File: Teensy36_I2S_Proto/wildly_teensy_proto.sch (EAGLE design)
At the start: 22 parts, among them CON1 MIKROE_BUS_CONN, SW1 SPST_TACT-KMR2, X1 ANTENNA

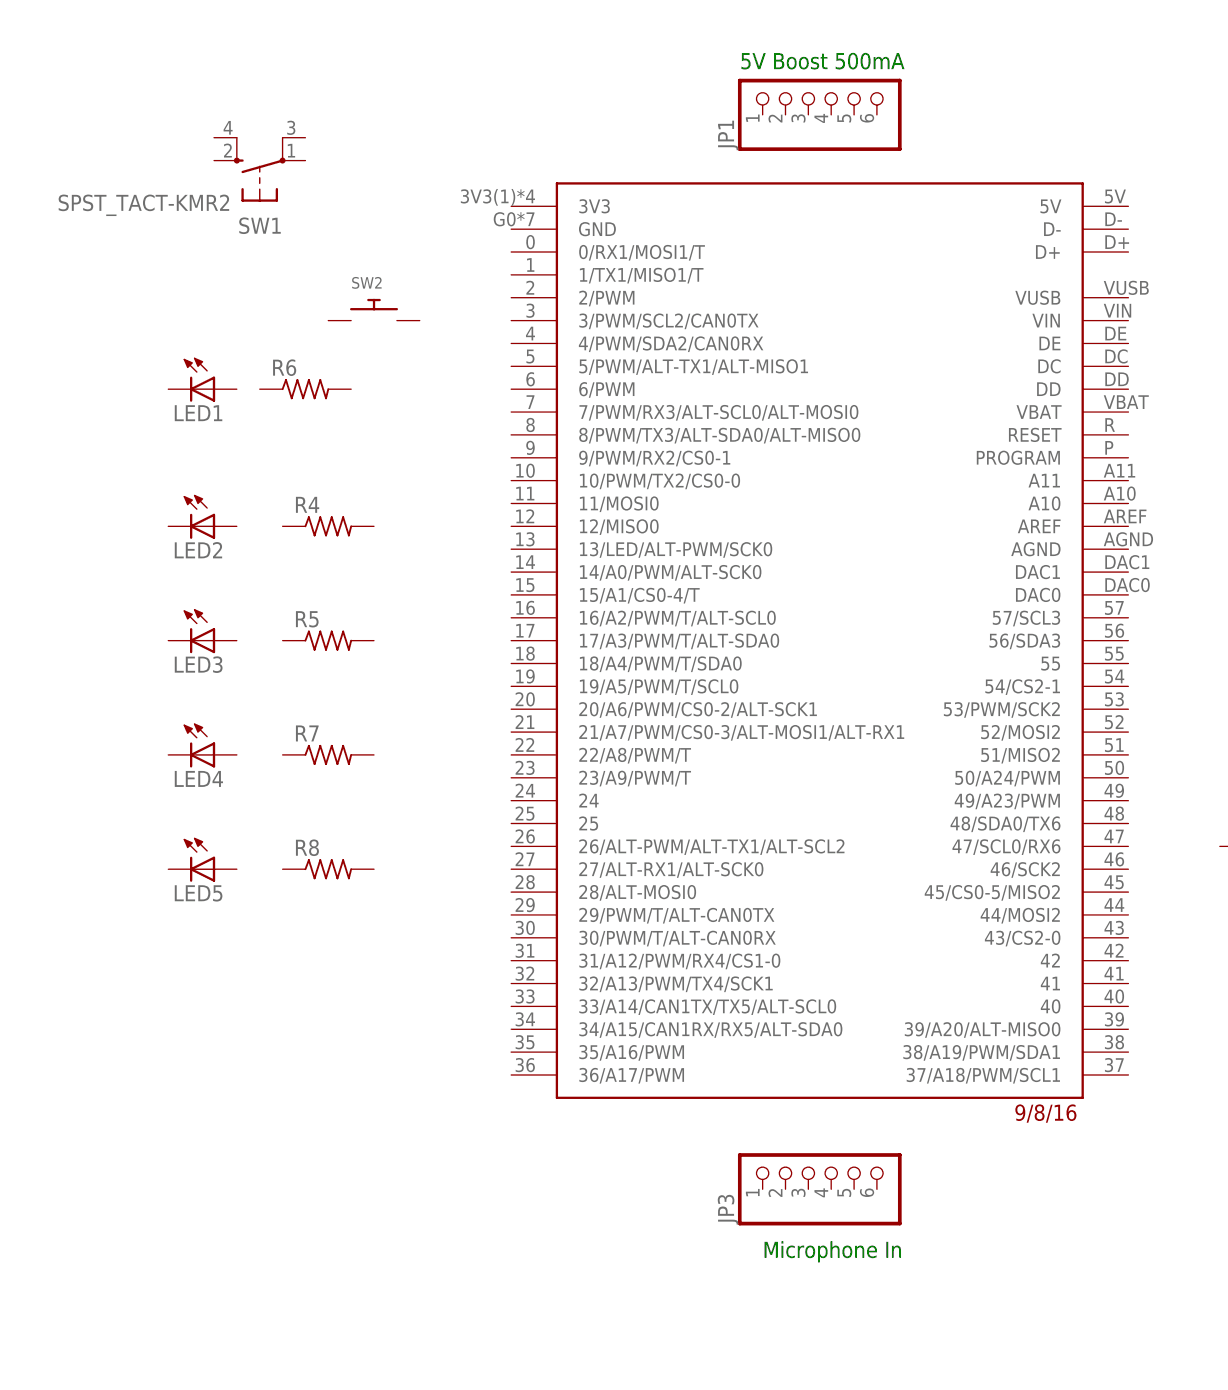
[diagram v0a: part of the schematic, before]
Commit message: Add files via upload
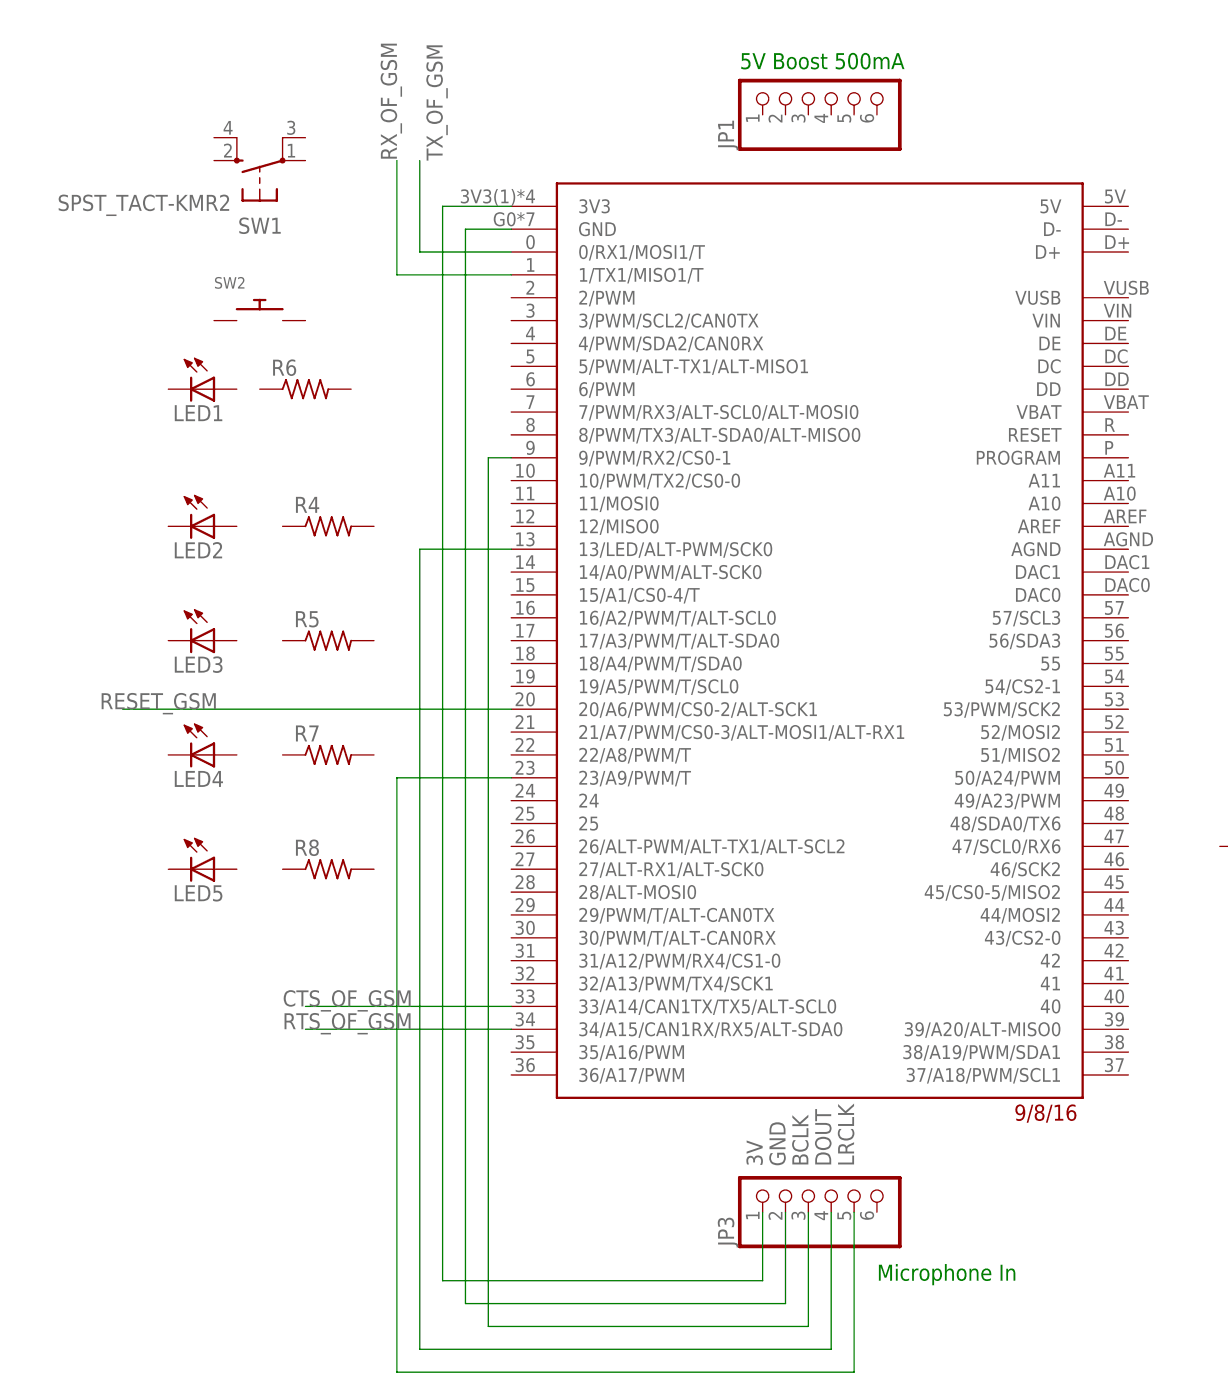
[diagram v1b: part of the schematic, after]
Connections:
- new net 3V: JP3.1, U$1.3V3
- new net BCLK: JP3.3, U$1.9/PWM/RX2/CS0-1
- new net CTS_OF_GSM: U$1.33/A14/CAN1TX/TX5/ALT-SCL0
- new net DOUT: JP3.4, U$1.13/LED/ALT-PWM/SCK0
- new net GND: JP3.2, U$1.GND
- new net LRCLK: JP3.5, U$1.23/A9/PWM/T
- new net RESET_GSM: U$1.20/A6/PWM/CS0-2/ALT-SCK1
- new net RTS_OF_GSM: U$1.34/A15/CAN1RX/RX5/ALT-SDA0
- new net RX_OF_GSM: U$1.1/TX1/MISO1/T
- new net TX_OF_GSM: U$1.0/RX1/MOSI1/T
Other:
- moved on the sheet: JP3, SW2
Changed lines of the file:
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@@
 <?xml version="1.0" encoding="utf-8"?>
 <!DOCTYPE eagle SYSTEM "eagle.dtd">
-<eagle version="9.3.0">
+<eagle version="9.2.2">
 <drawing>
 <settings>
@@
 <setting verticaltext="up"/>
 </settings>
-<grid distance="0.1" unitdist="inch" unit="inch" style="lines" multiple="1" display="no" altdistance="0.01" altunitdist="inch" altunit="inch"/>
+<grid distance="0.1" unitdist="inch" unit="inch" style="dots" multiple="1" display="yes" altdistance="0.01" altunitdist="inch" altunit="inch"/>
 <layers>
 <layer number="1" name="Top" color="4" fill="1" visible="no" active="no"/>
@@
 <sheet>
 <plain>
-<text x="58.42" y="-25.4" size="1.778" layer="91">Microphone In</text>
+<text x="71.12" y="-27.94" size="1.778" layer="91">Microphone In</text>
 <text x="55.88" y="106.68" size="1.778" layer="91">5V Boost 500mA</text>
 <text x="129.54" y="10.16" size="1.778" layer="91">5V Boost 1A</text>
@@
 <attribute name="VALUE" x="-0.635" y="92.71" size="1.778" layer="96" rot="R180"/>
 </instance>
-<instance part="SW2" gate="G$1" x="15.24" y="78.74" smashed="yes">
-<attribute name="NAME" x="12.7" y="82.296" size="1.27" layer="95"/>
-<attribute name="VALUE" x="12.7" y="76.454" size="1.27" layer="96"/>
+<instance part="SW2" gate="G$1" x="2.54" y="78.74" smashed="yes">
+<attribute name="NAME" x="-2.54" y="82.296" size="1.27" layer="95"/>
+<attribute name="VALUE" x="0" y="76.454" size="1.27" layer="96"/>
 </instance>
 <instance part="JP2" gate="G$1" x="137.16" y="15.24" smashed="yes" rot="R270">
@@
 <attribute name="VALUE" x="121.92" y="21.59" size="1.778" layer="96" rot="R270"/>
 </instance>
-<instance part="JP3" gate="A" x="66.04" y="-15.24" smashed="yes" rot="R90">
-<attribute name="NAME" x="55.245" y="-21.59" size="1.778" layer="95" rot="R90"/>
-<attribute name="VALUE" x="76.2" y="-21.59" size="1.778" layer="96" rot="R90"/>
+<instance part="JP3" gate="A" x="66.04" y="-17.78" smashed="yes" rot="R90">
+<attribute name="NAME" x="55.245" y="-24.13" size="1.778" layer="95" rot="R90"/>
+<attribute name="VALUE" x="76.2" y="-24.13" size="1.778" layer="96" rot="R90"/>
 </instance>
 <instance part="R8" gate="G$1" x="10.16" y="17.78" smashed="yes">
@@
 </segment>
 </net>
+<net name="3V" class="0">
+<segment>
+<pinref part="JP3" gate="A" pin="1"/>
+<wire x1="58.42" y1="-20.32" x2="58.42" y2="-27.94" width="0.1524" layer="91"/>
+<wire x1="58.42" y1="-27.94" x2="22.86" y2="-27.94" width="0.1524" layer="91"/>
+<wire x1="22.86" y1="-27.94" x2="22.86" y2="91.44" width="0.1524" layer="91"/>
+<pinref part="U$1" gate="G$1" pin="3V3"/>
+<wire x1="22.86" y1="91.44" x2="30.48" y2="91.44" width="0.1524" layer="91"/>
+<label x="58.42" y="-15.24" size="1.778" layer="95" rot="R90"/>
+</segment>
+</net>
+<net name="GND" class="0">
+<segment>
+<pinref part="JP3" gate="A" pin="2"/>
+<wire x1="60.96" y1="-20.32" x2="60.96" y2="-30.48" width="0.1524" layer="91"/>
+<wire x1="60.96" y1="-30.48" x2="25.4" y2="-30.48" width="0.1524" layer="91"/>
+<wire x1="25.4" y1="-30.48" x2="25.4" y2="88.9" width="0.1524" layer="91"/>
+<pinref part="U$1" gate="G$1" pin="GND"/>
+<wire x1="25.4" y1="88.9" x2="30.48" y2="88.9" width="0.1524" layer="91"/>
+<label x="60.96" y="-15.24" size="1.778" layer="95" rot="R90"/>
+</segment>
+</net>
+<net name="BCLK" class="0">
+<segment>
+<pinref part="JP3" gate="A" pin="3"/>
+<wire x1="63.5" y1="-20.32" x2="63.5" y2="-33.02" width="0.1524" layer="91"/>
+<wire x1="63.5" y1="-33.02" x2="27.94" y2="-33.02" width="0.1524" layer="91"/>
+<pinref part="U$1" gate="G$1" pin="9/PWM/RX2/CS0-1"/>
+<wire x1="27.94" y1="-33.02" x2="27.94" y2="63.5" width="0.1524" layer="91"/>
+<wire x1="27.94" y1="63.5" x2="30.48" y2="63.5" width="0.1524" layer="91"/>
+<label x="63.5" y="-15.24" size="1.778" layer="95" rot="R90"/>
+</segment>
+</net>
+<net name="DOUT" class="0">
+<segment>
+<pinref part="JP3" gate="A" pin="4"/>
+<wire x1="66.04" y1="-20.32" x2="66.04" y2="-35.56" width="0.1524" layer="91"/>
+<wire x1="66.04" y1="-35.56" x2="20.32" y2="-35.56" width="0.1524" layer="91"/>
+<pinref part="U$1" gate="G$1" pin="13/LED/ALT-PWM/SCK0"/>
+<wire x1="20.32" y1="-35.56" x2="20.32" y2="53.34" width="0.1524" layer="91"/>
+<wire x1="20.32" y1="53.34" x2="30.48" y2="53.34" width="0.1524" layer="91"/>
+<label x="66.04" y="-15.24" size="1.778" layer="95" rot="R90"/>
+</segment>
+</net>
+<net name="LRCLK" class="0">
+<segment>
+<pinref part="JP3" gate="A" pin="5"/>
+<wire x1="68.58" y1="-20.32" x2="68.58" y2="-38.1" width="0.1524" layer="91"/>
+<wire x1="68.58" y1="-38.1" x2="17.78" y2="-38.1" width="0.1524" layer="91"/>
+<wire x1="17.78" y1="-38.1" x2="17.78" y2="27.94" width="0.1524" layer="91"/>
+<label x="68.58" y="-15.24" size="1.778" layer="95" rot="R90"/>
+<pinref part="U$1" gate="G$1" pin="23/A9/PWM/T"/>
+<wire x1="17.78" y1="27.94" x2="30.48" y2="27.94" width="0.1524" layer="91"/>
+</segment>
+</net>
+<net name="TX_OF_GSM" class="0">
+<segment>
+<pinref part="U$1" gate="G$1" pin="0/RX1/MOSI1/T"/>
+<wire x1="30.48" y1="86.36" x2="20.32" y2="86.36" width="0.1524" layer="91"/>
+<wire x1="20.32" y1="86.36" x2="20.32" y2="96.52" width="0.1524" layer="91"/>
+<label x="22.86" y="96.52" size="1.778" layer="95" rot="R90"/>
+</segment>
+</net>
+<net name="RX_OF_GSM" class="0">
+<segment>
+<pinref part="U$1" gate="G$1" pin="1/TX1/MISO1/T"/>
+<wire x1="30.48" y1="83.82" x2="17.78" y2="83.82" width="0.1524" layer="91"/>
+<wire x1="17.78" y1="83.82" x2="17.78" y2="96.52" width="0.1524" layer="91"/>
+<label x="17.78" y="96.52" size="1.778" layer="95" rot="R90"/>
+</segment>
+</net>
+<net name="RESET_GSM" class="0">
+<segment>
+<pinref part="U$1" gate="G$1" pin="20/A6/PWM/CS0-2/ALT-SCK1"/>
+<wire x1="30.48" y1="35.56" x2="-12.7" y2="35.56" width="0.1524" layer="91"/>
+<label x="-15.24" y="35.56" size="1.778" layer="95"/>
+</segment>
+</net>
+<net name="CTS_OF_GSM" class="0">
+<segment>
+<pinref part="U$1" gate="G$1" pin="33/A14/CAN1TX/TX5/ALT-SCL0"/>
+<wire x1="30.48" y1="2.54" x2="7.62" y2="2.54" width="0.1524" layer="91"/>
+<label x="5.08" y="2.54" size="1.778" layer="95"/>
+</segment>
+</net>
+<net name="RTS_OF_GSM" class="0">
+<segment>
+<pinref part="U$1" gate="G$1" pin="34/A15/CAN1RX/RX5/ALT-SDA0"/>
+<wire x1="30.48" y1="0" x2="7.62" y2="0" width="0.1524" layer="91"/>
+<label x="5.08" y="0" size="1.778" layer="95"/>
+</segment>
+</net>

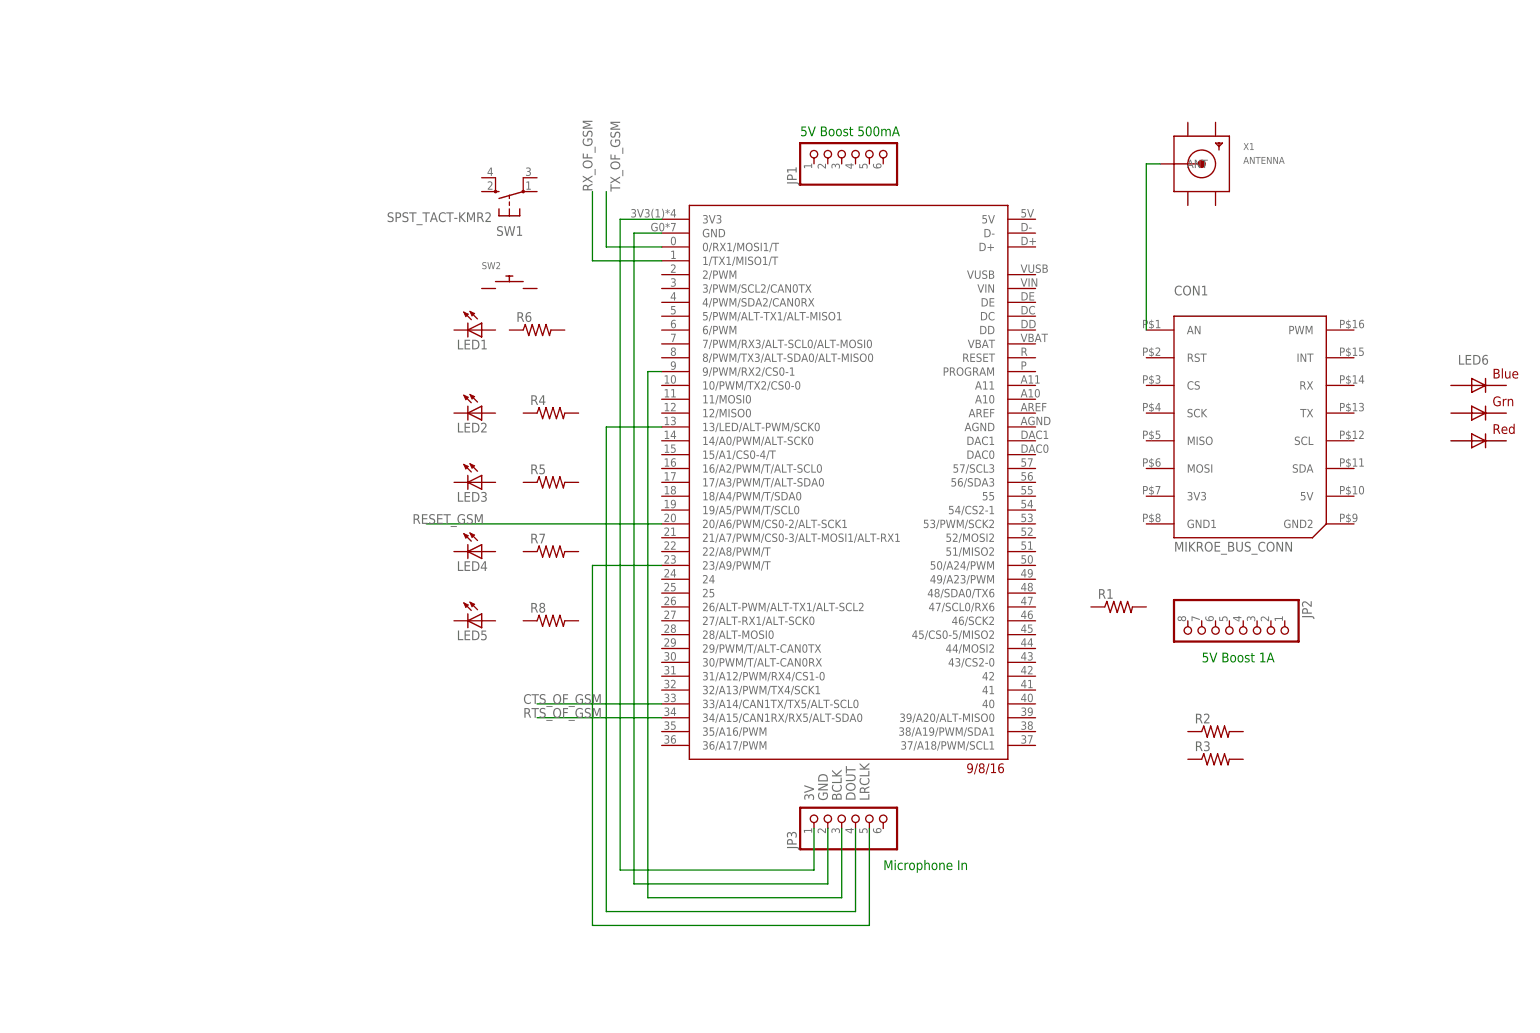
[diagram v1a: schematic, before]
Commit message: Add more connections to Teensy
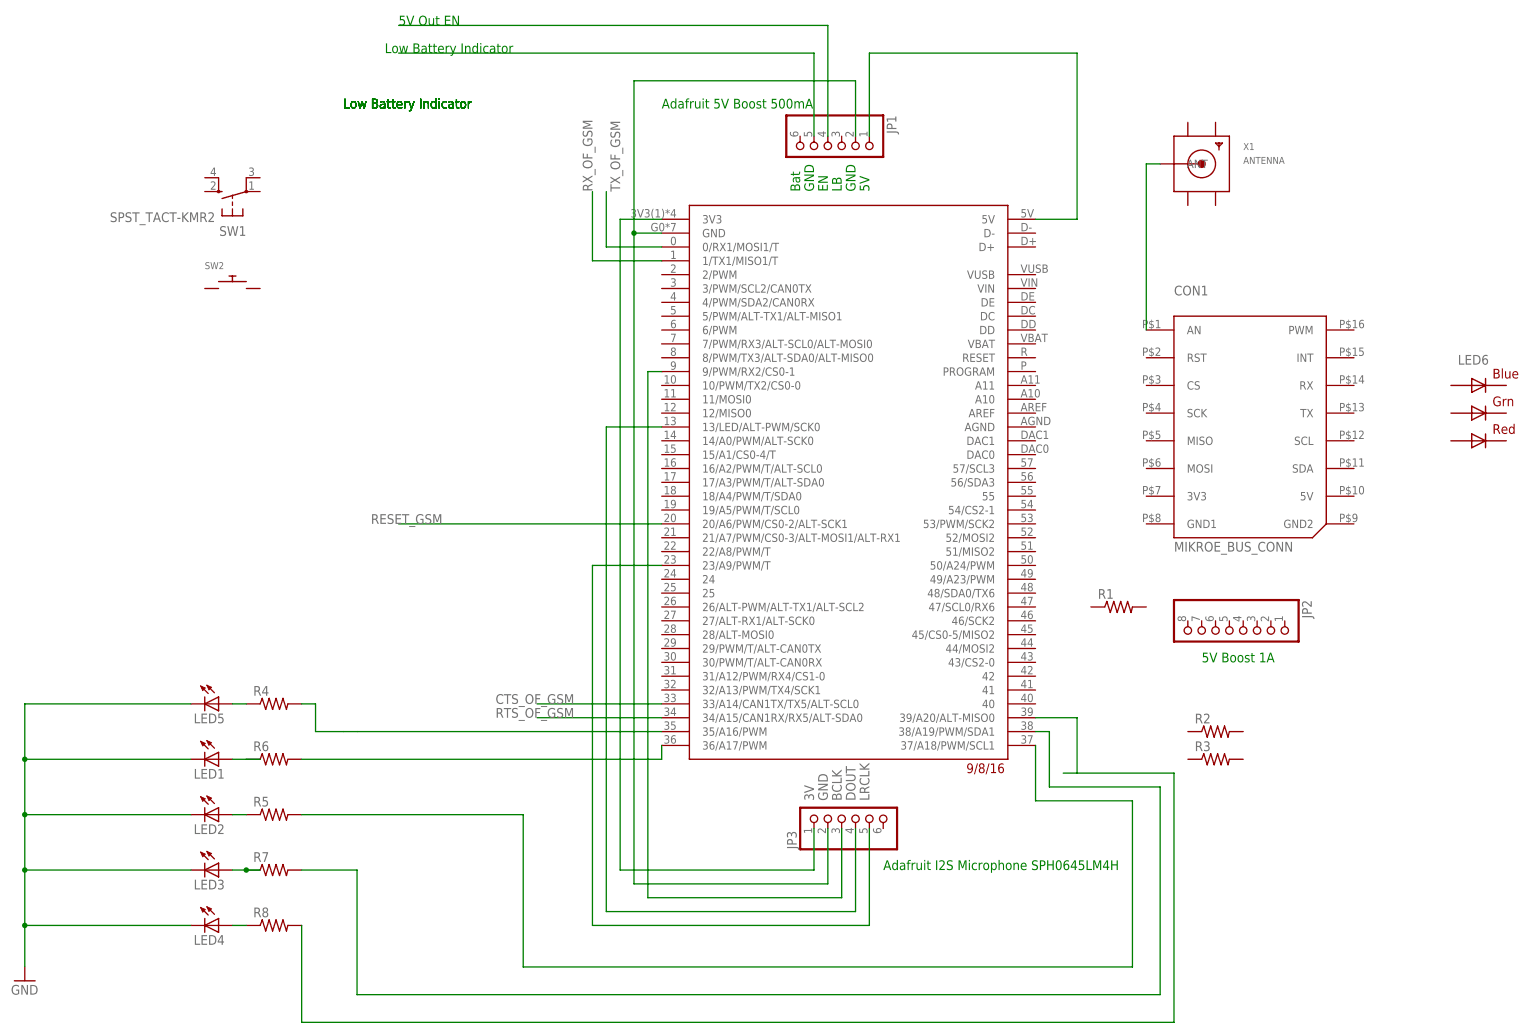
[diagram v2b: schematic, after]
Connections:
- new net N$11: LED3.A, R7.1
- new net N$12: LED2.A, R5.1
- new net N$13: R6.2, U$1.36/A17/PWM
- new net N$14: LED4.A, R8.1
- new net N$15: LED5.A, R4.1
- new net N$2: JP1.1, U$1.5V
- new net N$3: JP1.5
- new net N$4: JP1.4
- new net N$5: R4.2, U$1.35/A16/PWM
- new net N$6: R5.2, U$1.37/A18/PWM/SCL1
- new net N$7: R7.2, U$1.38/A19/PWM/SDA1
- new net N$8: R8.2, U$1.39/A20/ALT-MISO0
- new net N$9: LED1.A, R6.1
- net GND: now also JP1.2, LED1.C, LED2.C, LED3.C, LED4.C, LED5.C
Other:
- note added: "5V"
- note added: "5V Out EN"
- note added: "Adafruit 5V Boost 500mA"
- note added: "Adafruit I2S Microphone SPH0645LM4H"
- note added: "Bat"
- note added: "EN"
- note added: "GND"
- note added: "LB"
- note added: "Low Battery Indicator"
- note removed: "5V Boost 500mA"
- note removed: "Microphone In"
- moved on the sheet: JP1, LED1, LED2, LED3, LED4, LED5, R4, R5, R6, R7, R8, SW1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
